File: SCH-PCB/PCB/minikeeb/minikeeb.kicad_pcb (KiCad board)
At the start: 2 copper layers, 99.9 x 91 mm, 98 parts, among them J1 OLED, J2 Conn_01x02_Pin, J3 Conn_01x02_Pin, SW1 SW_PUSH-Lily58-cache, SW10 SW_PUSH-Lily58-cache, SW11 SW_PUSH-Lily58-cache, SW12 SW_PUSH-Lily58-cache, SW13 SW_PUSH-Lily58-cache, SW14 SW_PUSH-Lily58-cache, SW15 SW_PUSH-Lily58-cache, SW16 SW_PUSH-Lily58-cache, SW17 SW_PUSH-Lily58-cache, SW18 SW_PUSH-Lily58-cache, SW19 SW_PUSH-Lily58-cache, SW2 SW_PUSH-Lily58-cache, SW20 Rotary_Encoder_Switch-Device, SW3 SW_PUSH-Lily58-cache, SW4 SW_PUSH-Lily58-cache, SW5 SW_PUSH-Lily58-cache, SW6 SW_PUSH-Lily58-cache, SW7 SW_PUSH-Lily58-cache, SW8 SW_PUSH-Lily58-cache, SW9 SW_PUSH-Lily58-cache, U1 ProMicro_2-Lily58-cache, U2 TRRS

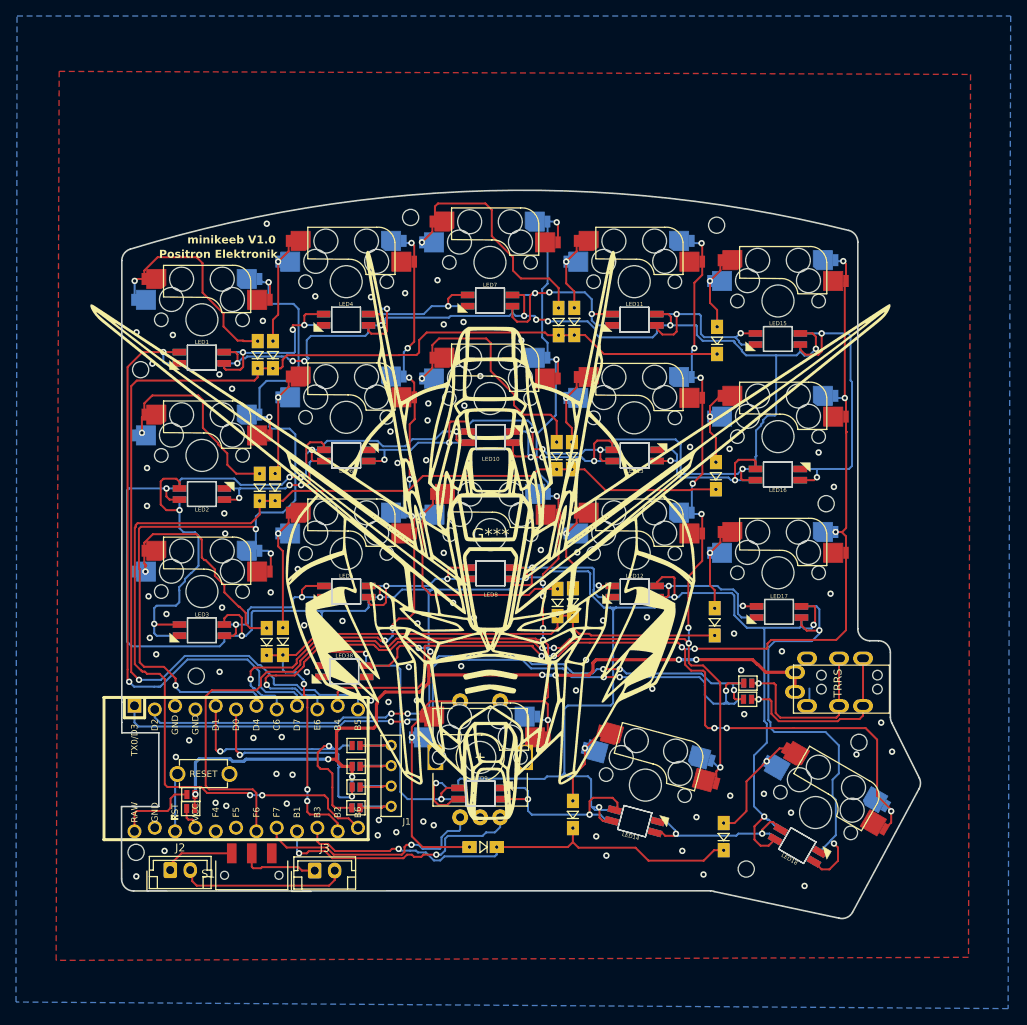
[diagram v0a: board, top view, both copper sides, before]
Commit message: FIX fix dimension PCB
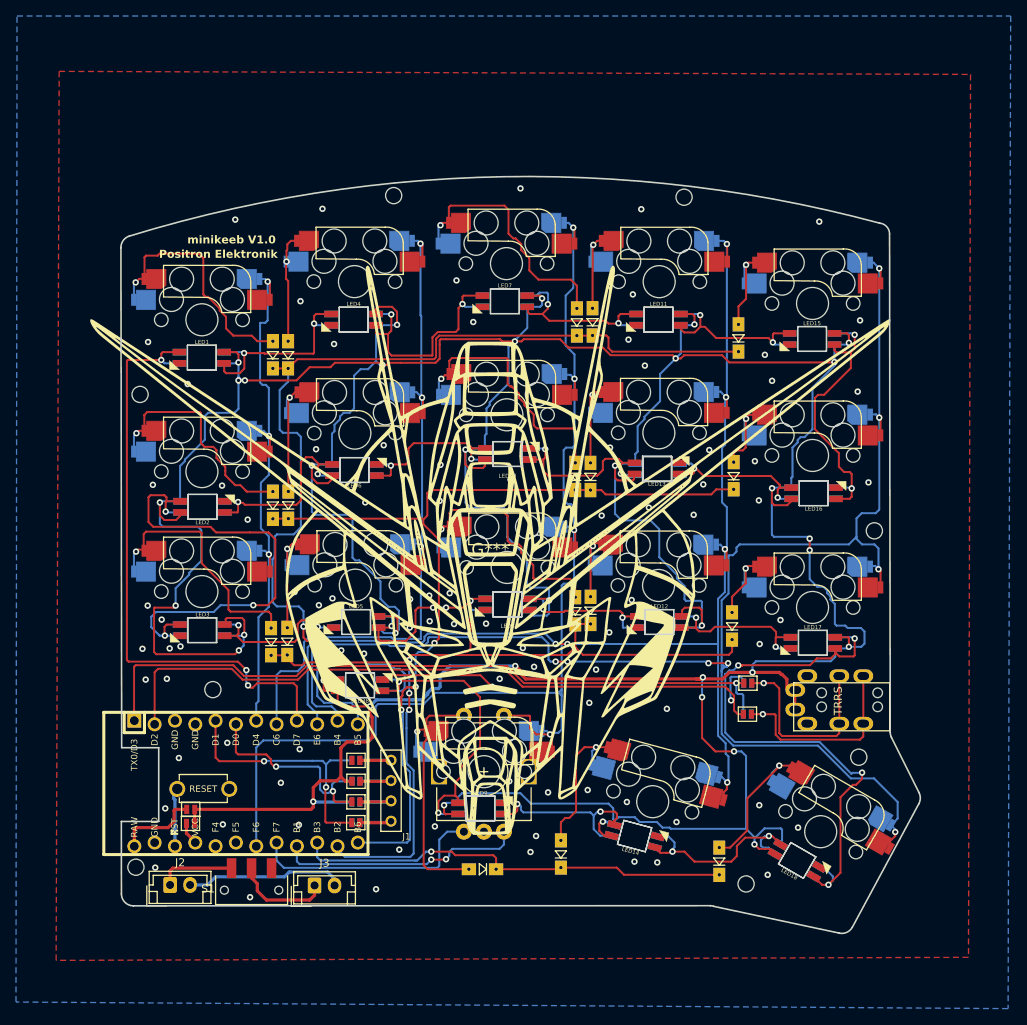
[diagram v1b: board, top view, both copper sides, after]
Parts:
- moved SW19 6.12 mm to (116.5, 119.1)
- moved LED17 5.73 mm to (116.5, 123.5)
- moved LED35 5.73 mm to (116.5, 123.5)
- moved D11 5.16 mm to (85.0, 149.9)
- moved LED16 5.04 mm to (116.6, 104.8)
- moved LED34 5.04 mm to (116.6, 104.8)
- moved SW15 5.02 mm to (97.2, 116.3)
- moved SW18 4.92 mm to (116.5, 100.1)
- moved LED12 4.89 mm to (97.3, 120.9)
- moved LED30 4.89 mm to (97.3, 120.9)
- moved SW11 4.60 mm to (78.3, 114.1)
- moved LED8 4.43 mm to (78.3, 118.7)
- moved LED26 4.43 mm to (78.3, 118.7)
- moved SW17 4.33 mm to (116.5, 81.1)
- moved LED33 4.27 mm to (116.4, 85.5)
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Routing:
- net VCC: track 598.3 -> 651.0 mm, vias 35 -> 36
- net col0: track 107.6 -> 68.3 mm, vias 5 -> 3
- net row1: track 139.7 -> 112.4 mm, vias 2 -> 3
- net row0: track 149.1 -> 122.1 mm, vias 1 -> 2
- net GND: track 1.49 -> 25.8 mm, vias 89 -> 90
- net col4: track 170.6 -> 193.6 mm, vias 10 -> 8
- net /10: track 37.8 -> 60.0 mm, vias 2 -> 3
- net row2: track 87.9 -> 102.0 mm
- net /15: track 57.1 -> 71.2 mm, vias 2 -> 4
- net /12: track 21.8 -> 33.1 mm, vias 2 -> 4
- net Net-(D11-A): track 10.2 -> 18.5 mm
- net col2: track 153.5 -> 146.0 mm, vias 8 -> 4
- net /2: track 23.9 -> 30.4 mm
- net col1: track 82.4 -> 88.1 mm, vias 8 -> 3
- net rxd0: track 94.2 -> 89.6 mm, vias 5 -> 1
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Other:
- board size 99.9 x 91 mm -> 99.9 x 94.6 mm
